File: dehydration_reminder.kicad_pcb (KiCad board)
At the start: 2 copper layers, 70 x 70 mm, 0 parts

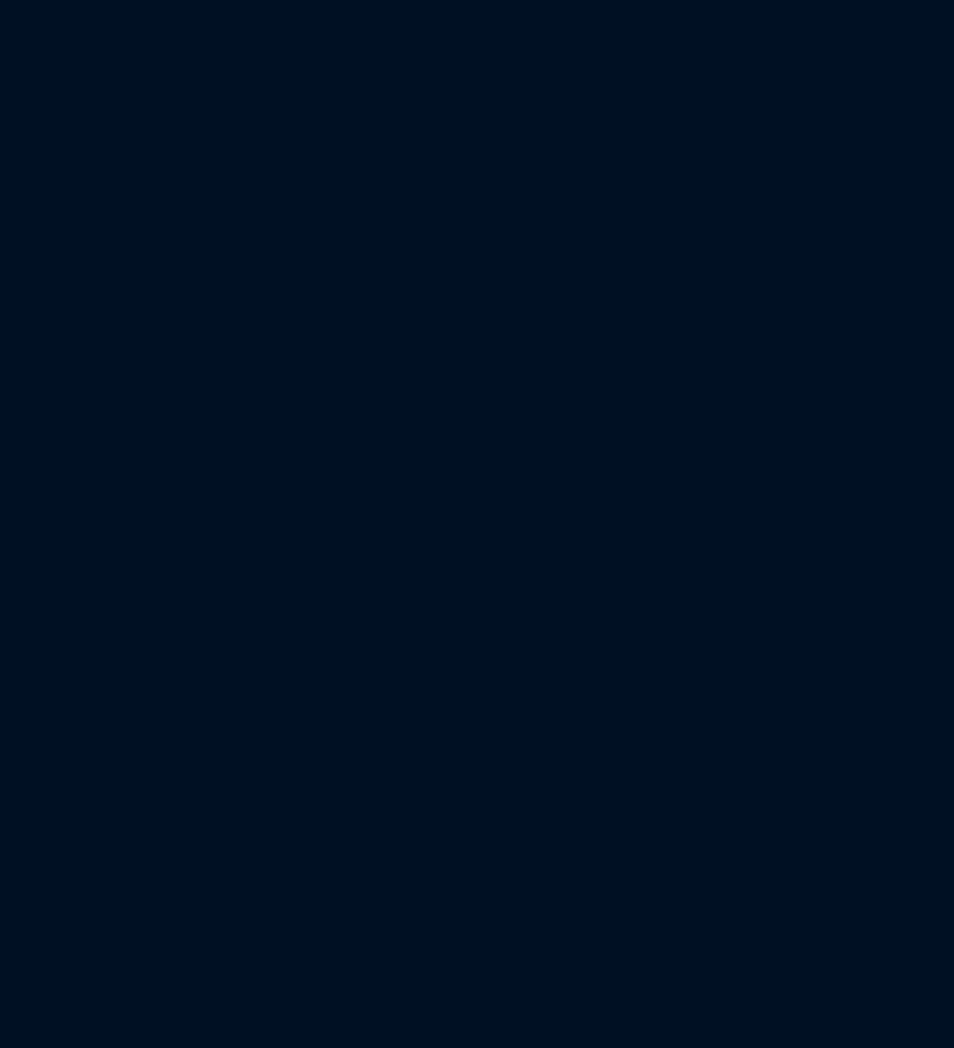
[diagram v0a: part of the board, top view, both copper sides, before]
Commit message: final schematic made and footprints assigned
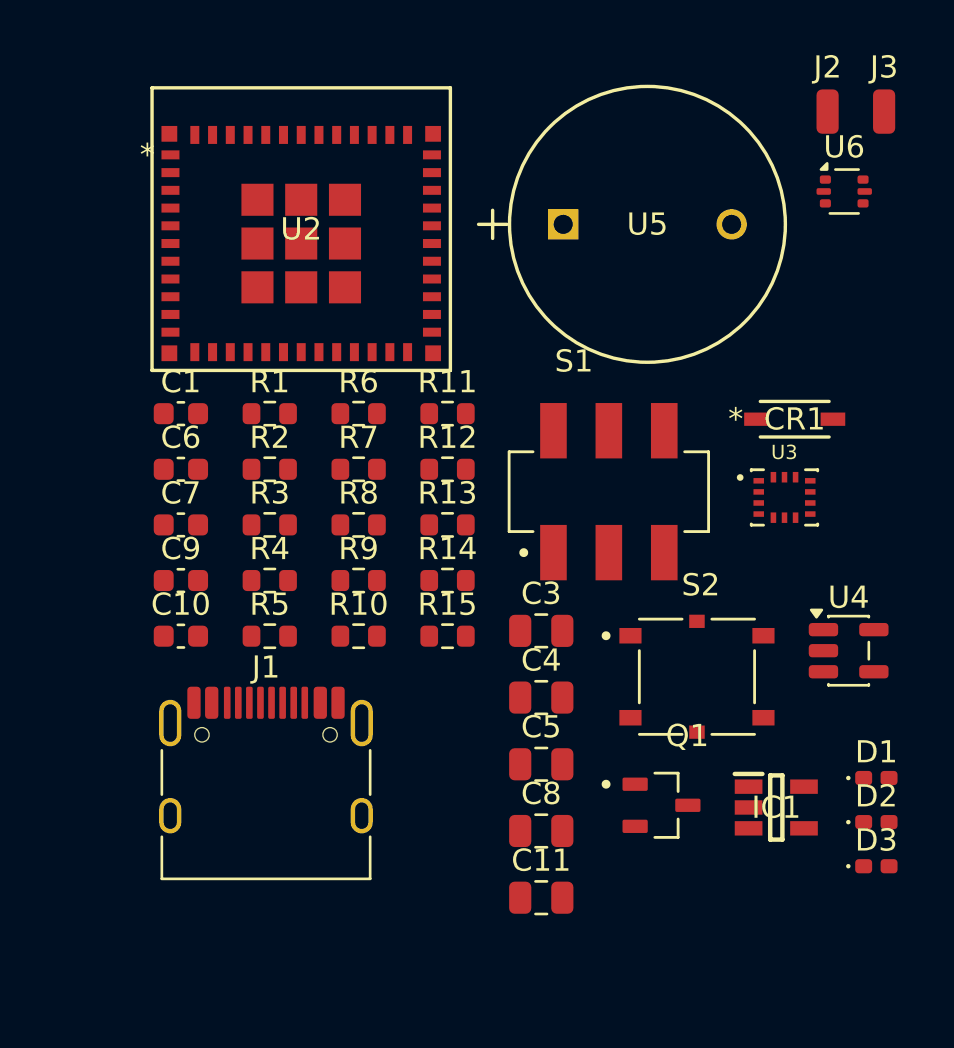
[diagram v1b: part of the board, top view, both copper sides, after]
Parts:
- added C1: 4.7nF, Capacitor_SMD:C_0603_1608Metric, F.Cu at (196.8, 55.6)
- added C10: 0.1uF, Capacitor_SMD:C_0603_1608Metric, F.Cu at (196.8, 65.7)
- added C11: 2.2uF, Capacitor_SMD:C_0805_2012Metric, F.Cu at (213.1, 77.5)
- added C3: 1uF, Capacitor_SMD:C_0805_2012Metric, F.Cu at (213.1, 65.4)
- added C4: 4.7uF, Capacitor_SMD:C_0805_2012Metric, F.Cu at (213.1, 68.4)
- added C5: 4.7uF, Capacitor_SMD:C_0805_2012Metric, F.Cu at (213.1, 71.5)
- added C6: 100nF, Capacitor_SMD:C_0603_1608Metric, F.Cu at (196.8, 58.1)
- added C7: 100nF, Capacitor_SMD:C_0603_1608Metric, F.Cu at (196.8, 60.6)
- added C8: 1uF, Capacitor_SMD:C_0805_2012Metric, F.Cu at (213.1, 74.5)
- added C9: 0.1uF, Capacitor_SMD:C_0603_1608Metric, F.Cu at (196.8, 63.2)
- added CR1: 1N4148W-7-F, footprints2:SOD123_DIO, F.Cu at (224.5, 55.9)
- added D1: BLUE LED, LED_SMD:LED_0402_1005Metric_Pad0.77x0.64mm_HandSolder, F.Cu at (228.2, 72.1)
- added D2: RED LED, LED_SMD:LED_0402_1005Metric_Pad0.77x0.64mm_HandSolder, F.Cu at (228.2, 74.1)
- added D3: GREEN LED, LED_SMD:LED_0402_1005Metric_Pad0.77x0.64mm_HandSolder, F.Cu at (228.2, 76.0)
- added IC1: RT9080-33GJ5, RT9080-33GJ5:SOT94P280X100-5N, F.Cu at (223.7, 73.4)
- added J1: USB_C_Receptacle_USB2.0_16P, Connector_USB:USB_C_Receptacle_HRO_TYPE-C-31-M-12, F.Cu at (200.7, 72.7)
- added J2: BAT-, Connector_Wire:SolderWirePad_1x01_SMD_1x2mm, F.Cu at (226.0, 42.0)
- added J3: BAT+, Connector_Wire:SolderWirePad_1x01_SMD_1x2mm, F.Cu at (228.6, 42.0)
- added Q1: AO3400-5.8A, AO3400-5.8A:SOT95P260X140-3N, F.Cu at (218.5, 73.3)
- added R1: 5.1K, Resistor_SMD:R_0603_1608Metric, F.Cu at (200.8, 55.6)
- added R10: 10K, Resistor_SMD:R_0603_1608Metric, F.Cu at (204.8, 65.7)
- added R11: 100, Resistor_SMD:R_0603_1608Metric, F.Cu at (208.9, 55.6)
- added R12: 50, Resistor_SMD:R_0603_1608Metric, F.Cu at (208.9, 58.1)
- added R13: 100K, Resistor_SMD:R_0603_1608Metric, F.Cu at (208.9, 60.6)
- added R14: 100K, Resistor_SMD:R_0603_1608Metric, F.Cu at (208.9, 63.2)
- added R15: 100K, Resistor_SMD:R_0603_1608Metric, F.Cu at (208.9, 65.7)
- added R2: 5.1K, Resistor_SMD:R_0603_1608Metric, F.Cu at (200.8, 58.1)
- added R3: 1M, Resistor_SMD:R_0603_1608Metric, F.Cu at (200.8, 60.6)
- added R4: 4.7K, Resistor_SMD:R_0603_1608Metric, F.Cu at (200.8, 63.2)
- added R5: 120k, Resistor_SMD:R_0603_1608Metric, F.Cu at (200.8, 65.7)
- added R6: 10K, Resistor_SMD:R_0603_1608Metric, F.Cu at (204.8, 55.6)
- added R7: 4.7K, Resistor_SMD:R_0603_1608Metric, F.Cu at (204.8, 58.1)
- added R8: 4.7K, Resistor_SMD:R_0603_1608Metric, F.Cu at (204.8, 60.6)
- added R9: 10K, Resistor_SMD:R_0603_1608Metric, F.Cu at (204.8, 63.2)
- added S1: JS202011SCQN, JS202011SCQN:SW_JS202011SCQN, F.Cu at (216.1, 59.1)
- added S2: PTS526_SMG15_SMTR2_LFS, PTS526_SMG15_SMTR2_LFS:SW_PTS526_SMG15_SMTR2_LFS, F.Cu at (220.1, 67.5)
- added U2: ESP32-C3-MINI-1U-H4, footprints3:ESP32-C3-MINI-1U_EXP, F.Cu at (202.3, 47.3)
- added U3: BMI270, BMI270:XDCR_BMI270, F.Cu at (224.1, 59.4)
- added U4: MCP73831-2-OT, Package_TO_SOT_SMD:SOT-23-5, F.Cu at (227.0, 66.3)
- added U5: TMB12A03, footprints4:AUDIO_TMB12A03_JHE, F.Cu at (214.1, 47.1)
- added U6: USBLC6-2P6, Package_TO_SOT_SMD:SOT-666, F.Cu at (226.8, 45.6)

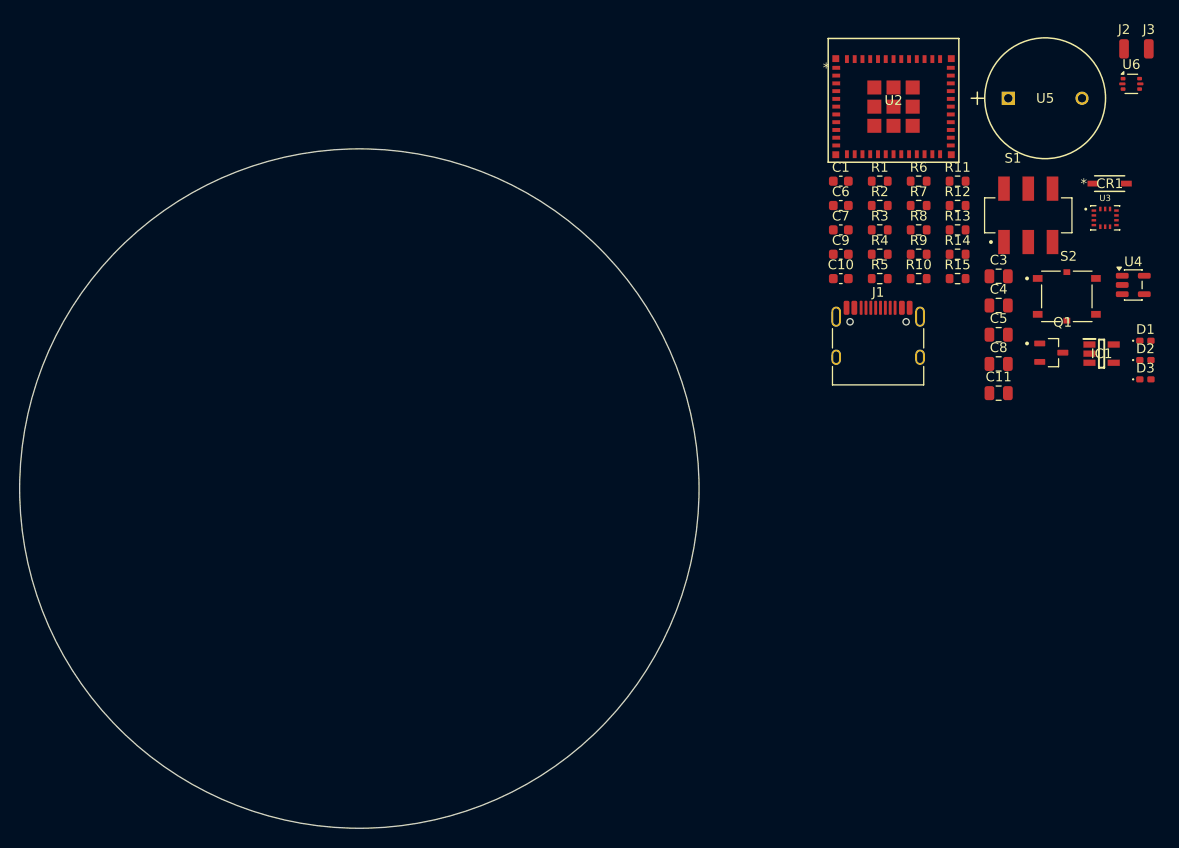
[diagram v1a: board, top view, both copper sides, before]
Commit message: first iteration of pcb ready
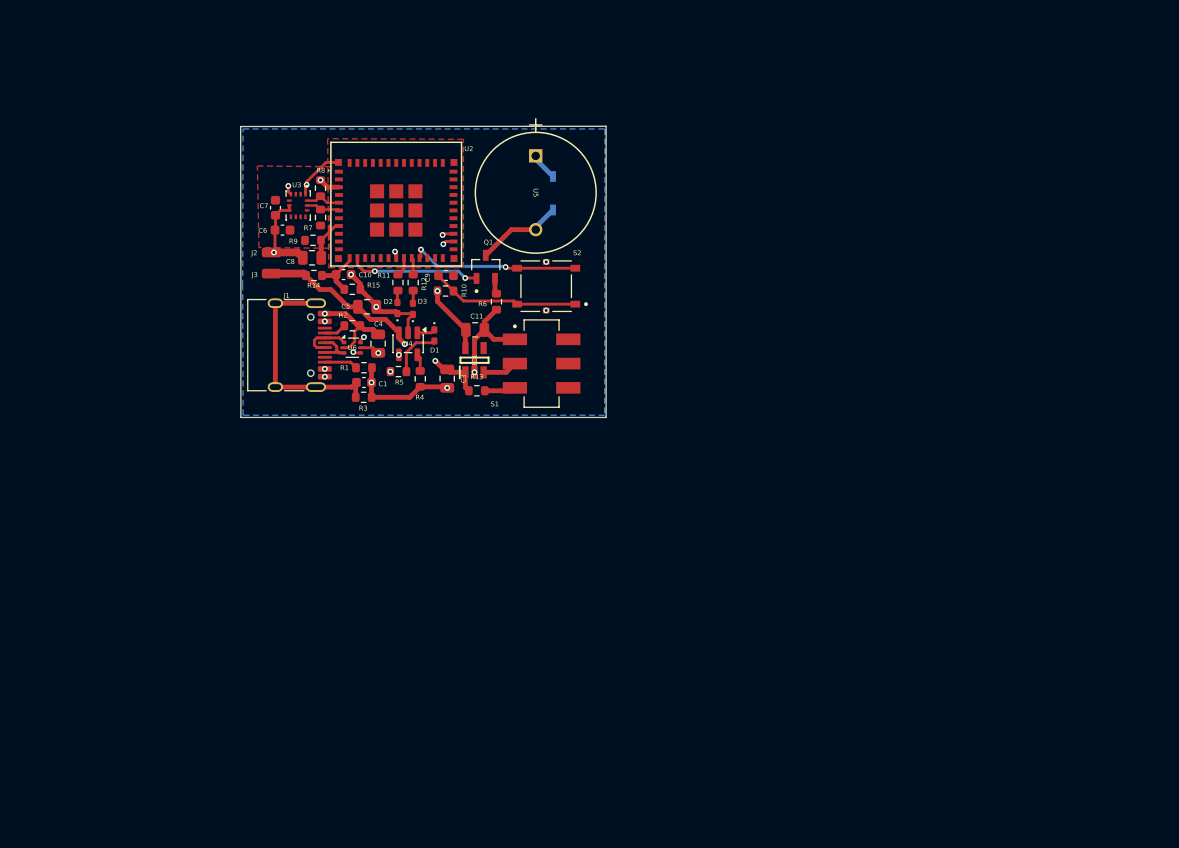
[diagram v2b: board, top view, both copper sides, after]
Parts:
- CR1: moved to B.Cu
- moved J3 93.3 mm to (138.2, 65.2), turned to 90 degrees
- moved J2 90.3 mm to (138.2, 63.0), turned to 90 degrees
- moved U6 84.7 mm to (146.5, 72.8)
- moved U3 83.1 mm to (140.9, 58.1), turned to -90 degrees
- moved D2 77.2 mm to (151.2, 68.7), turned to 90 degrees
- moved D3 75.8 mm to (152.7, 68.8), turned to 90 degrees
- moved U4 75.0 mm to (152.2, 72.4), turned to -90 degrees
- moved D1 73.3 mm to (154.9, 71.5), turned to -90 degrees
- moved C8 71.6 mm to (142.3, 63.5), turned to 180 degrees
- moved R14 66.3 mm to (142.6, 65.3)
- moved C5 65.1 mm to (148.0, 68.6)
- moved IC1 64.6 mm to (159.1, 74.1), turned to 90 degrees
- moved C4 64.1 mm to (149.2, 72.4), turned to 90 degrees
- moved R9 62.4 mm to (142.4, 61.7)
- moved R15 62.4 mm to (146.5, 66.8)
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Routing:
- net GND: track 0.00 -> 57.6 mm, vias 0 -> 11
- net Net-(IC1-VIN): track 0.00 -> 26.6 mm, vias 0 -> 2
- net Net-(J1-SHIELD): track 0.00 -> 22.9 mm
- net /USB_DP: track 0.00 -> 17.8 mm, vias 0 -> 2
- net /USB_DN: track 0.00 -> 17.7 mm, vias 0 -> 2
- net Net-(U2-IO7): track 0.00 -> 17.6 mm, vias 0 -> 2
- net /INT1: track 0.00 -> 15.5 mm, vias 0 -> 2
- net Net-(C9-Pad1): track 0.00 -> 15.4 mm
- net /BUZZ: track 0.00 -> 13.6 mm, vias 0 -> 2
- net /3.3v: track 0.00 -> 12.4 mm, vias 0 -> 2
- net Net-(CR1-Pad2): track 0.00 -> 9.01 mm
- net /ADC: track 0.00 -> 5.65 mm
- net Net-(D1-A): track 0.00 -> 5.34 mm
- net Net-(J1-D--PadA7): track 0.00 -> 5.04 mm
- net Net-(U2-EN): track 0.00 -> 4.27 mm
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- added copper zone on F.Cu, net /3.3v
- added copper zone on In1.Cu, net /3.3v
- added copper zone on In1.Cu, net /5V
- added copper zone on B.Cu, net GND
- added copper zone on F.Cu, net GND
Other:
- board size 70 x 70 mm -> 37.7 x 30 mm
- copper layers 2 -> 4
